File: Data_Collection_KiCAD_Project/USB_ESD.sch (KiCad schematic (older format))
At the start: 9 parts, among them J1 USB_B_Micro, U1 LM317T, U2 USBLC6-2SC6

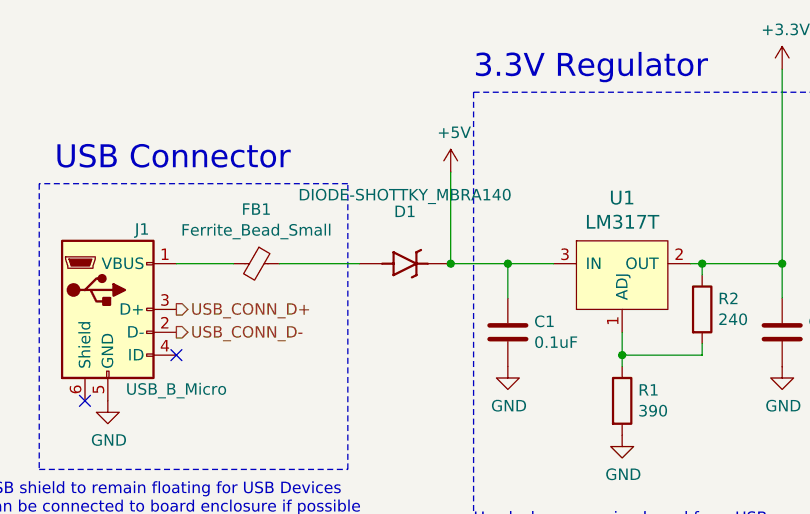
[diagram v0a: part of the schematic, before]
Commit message: Finalized Schematic
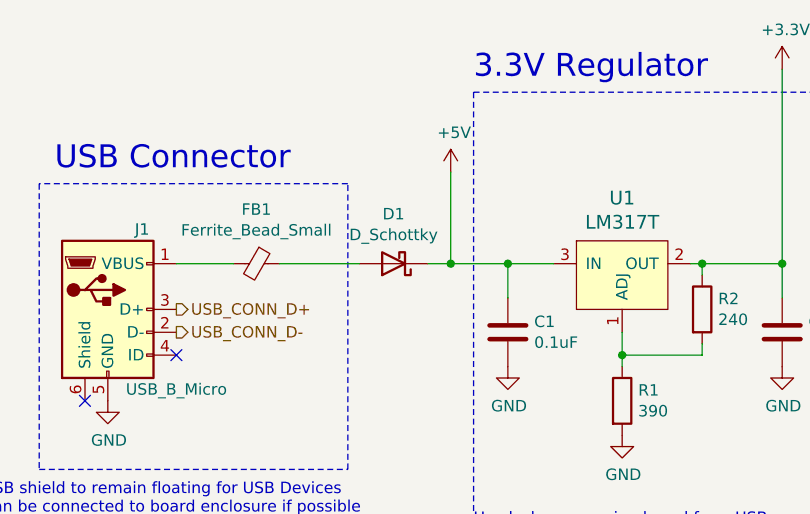
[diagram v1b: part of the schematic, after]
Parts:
- removed D1: DIODE-SHOTTKY_MBRA140, Silicon-Standard:SMA-DIODE, symbol SparkFun-DiscreteSemi:DIODE-SHOTTKY_MBRA140
- added D1: D_Schottky, Diode_SMD:D_0603_1608Metric, symbol Device:D_Schottky
- FB1: footprint (none) -> Capacitor_SMD:C_0603_1608Metric
- J1: footprint (none) -> Connector_USB:USB_Micro-B_Amphenol_10103594-0001LF_Horizontal
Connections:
- net +5V: now also D1.1 (K)
- net at FB1.1: now also D1.2 (A)
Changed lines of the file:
@@
 F 0 "J1" H 2300 4300 50  0000 C CNN
 F 1 "USB_B_Micro" H 2450 3600 50  0000 C CNN
-F 2 "" H 2300 3900 50  0001 C CNN
+F 2 "Connector_USB:USB_Micro-B_Amphenol_10103594-0001LF_Horizontal" H 2300 3900 50  0001 C CNN
 F 3 "~" H 2300 3900 50  0001 C CNN
 	1    2150 3950
@@
 F 0 "FB1" V 2563 3750 50  0000 C CNN
 F 1 "Ferrite_Bead_Small" V 2654 3750 50  0000 C CNN
-F 2 "" V 2730 3750 50  0001 C CNN
+F 2 "Capacitor_SMD:C_0603_1608Metric" V 2730 3750 50  0001 C CNN
 F 3 "~" H 2800 3750 50  0001 C CNN
 	1    2800 3750
@@
 Wire Wire Line
 	5100 2900 5100 3750
-$Comp
-L SparkFun-DiscreteSemi:DIODE-SHOTTKY_MBRA140 D1
-U 1 1 61A08B7E
-P 3450 3750
-F 0 "D1" H 3450 3977 50  0000 C CNN
-F 1 "DIODE-SHOTTKY_MBRA140" H 3450 4050 50  0000 C CNN
-F 2 "Silicon-Standard:SMA-DIODE" H 4100 3600 50  0001 C CNN
-F 3 "" H 3450 3750 50  0001 C CNN
-F 4 "DIO-08053" H 3450 3885 50  0001 C CNN "Field4"
-	1    3450 3750
-	1    0    0    -1
-$EndComp
 Wire Wire Line
 	3650 3350 3650 3750
@@
 Wire Wire Line
 	3650 3750 3900 3750
+Connection ~ 3900 3750
+$Comp
+L Device:D_Schottky D1
+U 1 1 61B1913C
+P 3400 3750
+F 0 "D1" H 3400 3533 50  0000 C CNN
+F 1 "D_Schottky" H 3400 3624 50  0000 C CNN
+F 2 "Diode_SMD:D_0603_1608Metric" H 3400 3750 50  0001 C CNN
+F 3 "~" H 3400 3750 50  0001 C CNN
+	1    3400 3750
+	-1   0    0    1
+$EndComp
+Wire Wire Line
+	3550 3750 3650 3750
 Connection ~ 3650 3750
-Connection ~ 3900 3750
 $EndSCHEMATC
